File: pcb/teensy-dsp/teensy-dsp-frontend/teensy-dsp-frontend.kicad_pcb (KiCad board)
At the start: 4 copper layers, 88 x 75 mm, 18 parts, among them J1 Conn_02x15_Odd_Even, U1 TLC5940PWP

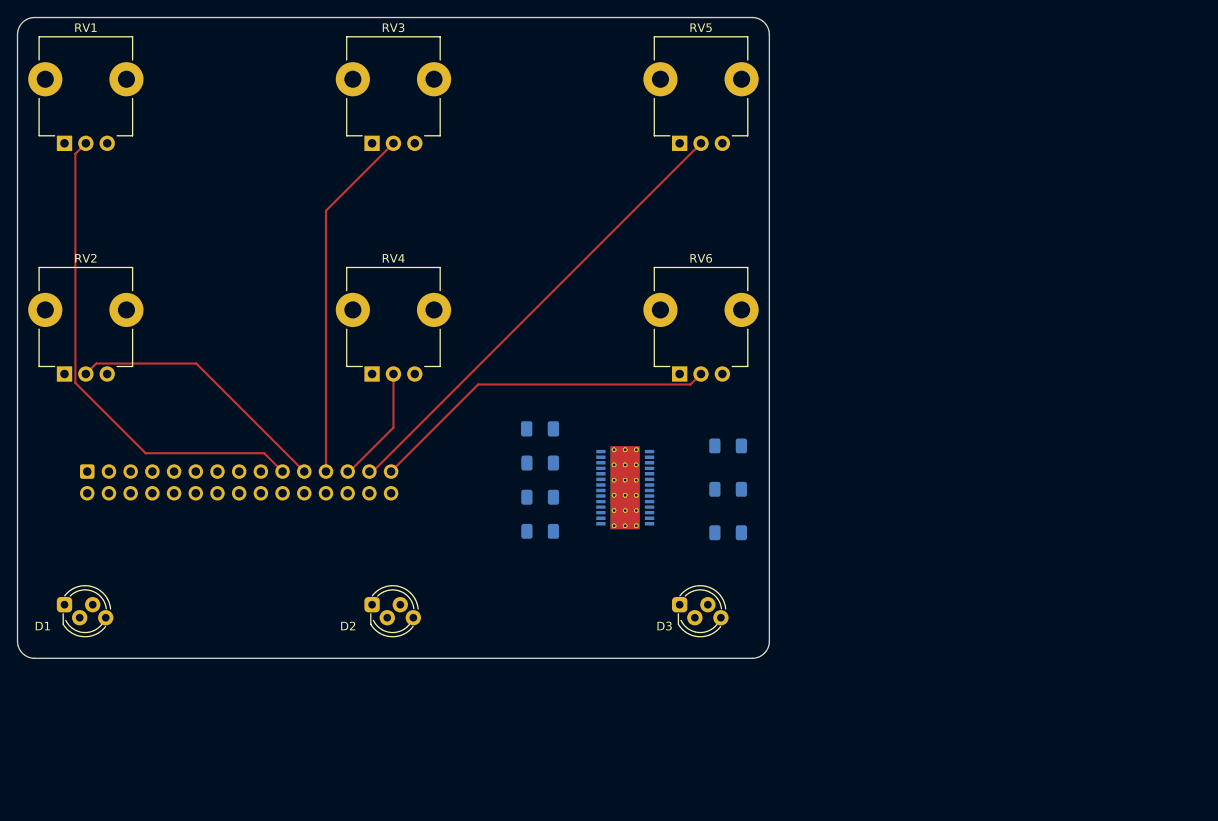
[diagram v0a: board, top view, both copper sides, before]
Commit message: pcb and case updates
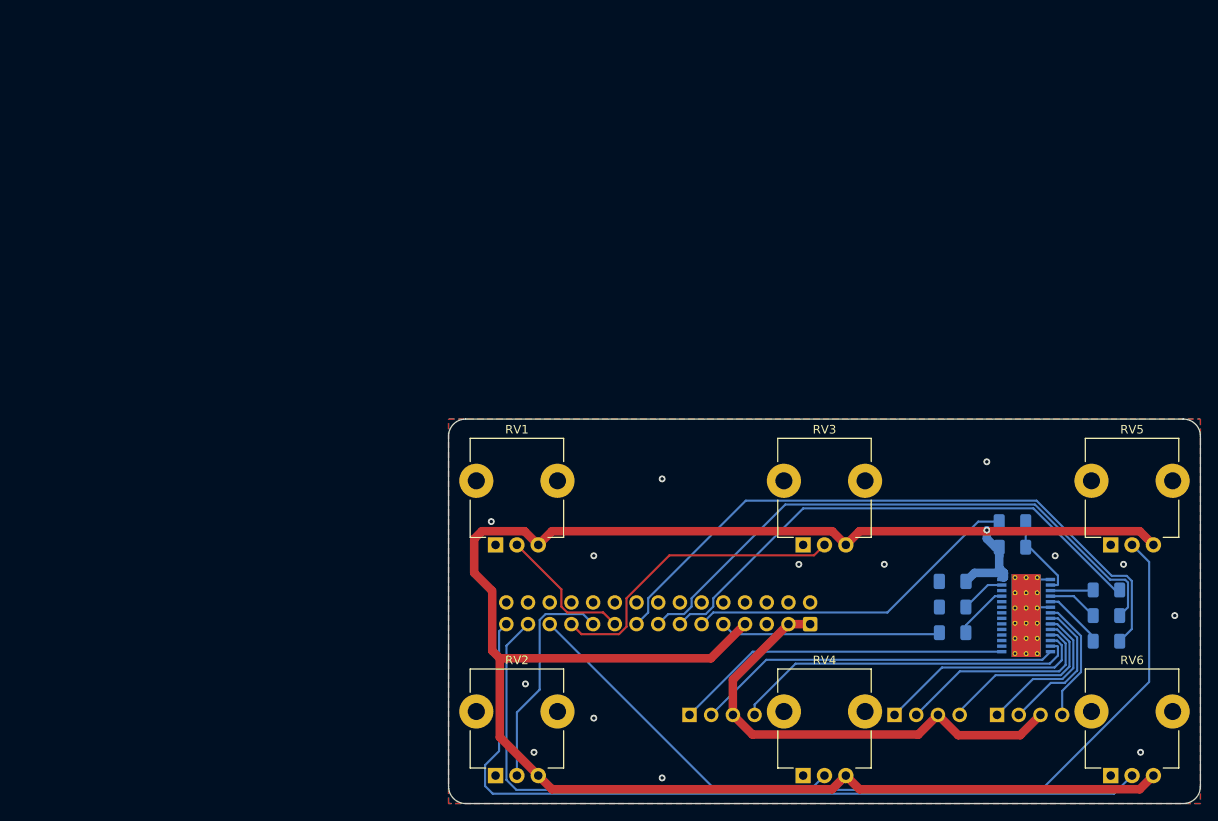
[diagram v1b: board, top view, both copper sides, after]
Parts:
- removed D1, D2, D3: LED_RABG, LED_THT:LED_D5.0mm-4_RGB_Staggered_Pins
- added J2: Conn_01x04_Pin, Connector_PinHeader_2.54mm:PinHeader_1x04_P2.54mm_Horizontal, B.Cu at (166.7, 112.6)
- added J3: Conn_01x04_Pin, Connector_PinHeader_2.54mm:PinHeader_1x04_P2.54mm_Horizontal, B.Cu at (154.7, 112.6)
- added J4: Conn_01x04_Pin, Connector_PinHeader_2.54mm:PinHeader_1x04_P2.54mm_Horizontal, B.Cu at (130.7, 112.6)
- added R7: 10k, Resistor_SMD:R_1206_3216Metric_Pad1.30x1.75mm_HandSolder, B.Cu at (168.4, 93.0)
- moved J1 86.5 mm to (144.8, 102.0), turned to 90 degrees
- moved RV1 69.0 mm to (108.0, 92.7)
- moved RV2 69.0 mm to (108.0, 119.7)
- moved RV4 69.0 mm to (143.9, 119.7)
- moved RV6 69.0 mm to (179.9, 119.7)
- moved RV3 69.0 mm to (143.9, 92.7)
- moved RV5 69.0 mm to (179.9, 92.7)
- moved R3 55.3 mm to (168.4, 90.0)
- moved C1 51.5 mm to (161.4, 97.0), turned to 0 degrees
- moved R1 51.1 mm to (161.4, 100.0)
- moved R2 50.8 mm to (161.4, 103.0)
- moved R6 49.8 mm to (179.4, 104.0), turned to 0 degrees
- moved U1 49.3 mm to (170.1, 101.0)
- moved R5 46.7 mm to (179.4, 101.0), turned to 0 degrees
- moved R4 44.8 mm to (179.4, 98.0), turned to 0 degrees
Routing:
- net +3.3V: track 0.00 -> 230.6 mm, vias 0 -> 1
- net LED_SIN: track 0.00 -> 76.5 mm
- net LED_SCLK: track 0.00 -> 69.4 mm
- net POT_5: track 54.7 -> 117.1 mm
- net LED_XLAT: track 0.00 -> 61.6 mm
- net POT_6: track 41.1 -> 97.0 mm
- net +9V: track 0.00 -> 55.7 mm
- net Net-(J4-Pin_2): track 0.00 -> 42.8 mm
- net Net-(J4-Pin_4): track 0.00 -> 41.0 mm
- net POT_1: track 57.1 -> 16.5 mm
- net Net-(J4-Pin_1): track 0.00 -> 39.6 mm
- net LED_BLANK: track 0.00 -> 39.4 mm
- net POT_4: track 14.1 -> 40.5 mm
- net LED_GSCLK: track 0.00 -> 25.8 mm
- net Net-(J3-Pin_1): track 0.00 -> 25.5 mm
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- added copper zone on B.Cu, net GND
- added copper zone on F.Cu, net GND
- removed copper zone on In2.Cu, net +3.3V
- removed copper zone on In2.Cu, net +9V
- removed copper zone on In1.Cu, net GND
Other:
- board size 88 x 75 mm -> 88 x 45 mm
- copper layers 4 -> 2
